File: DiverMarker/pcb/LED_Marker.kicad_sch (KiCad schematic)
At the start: 27 parts, among them IC101 PIC16LF15313, J101 SKEDD6, Q100 BST-52, Q101 BST-52, SW101 MK15-C2

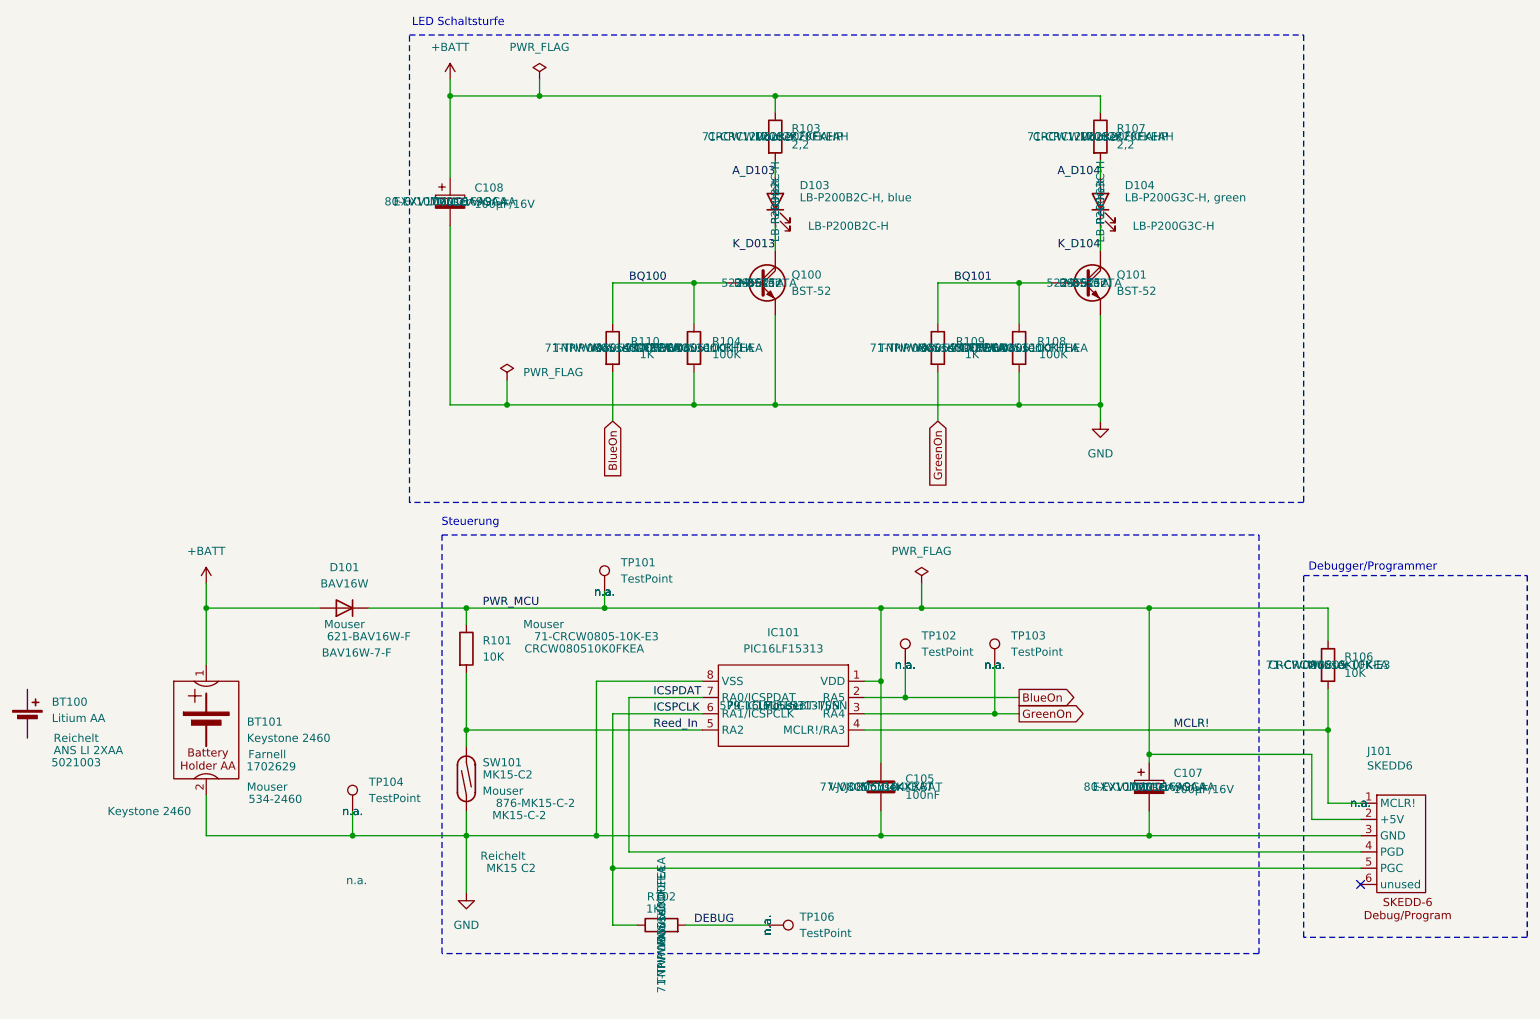
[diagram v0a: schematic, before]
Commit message: Working on BON
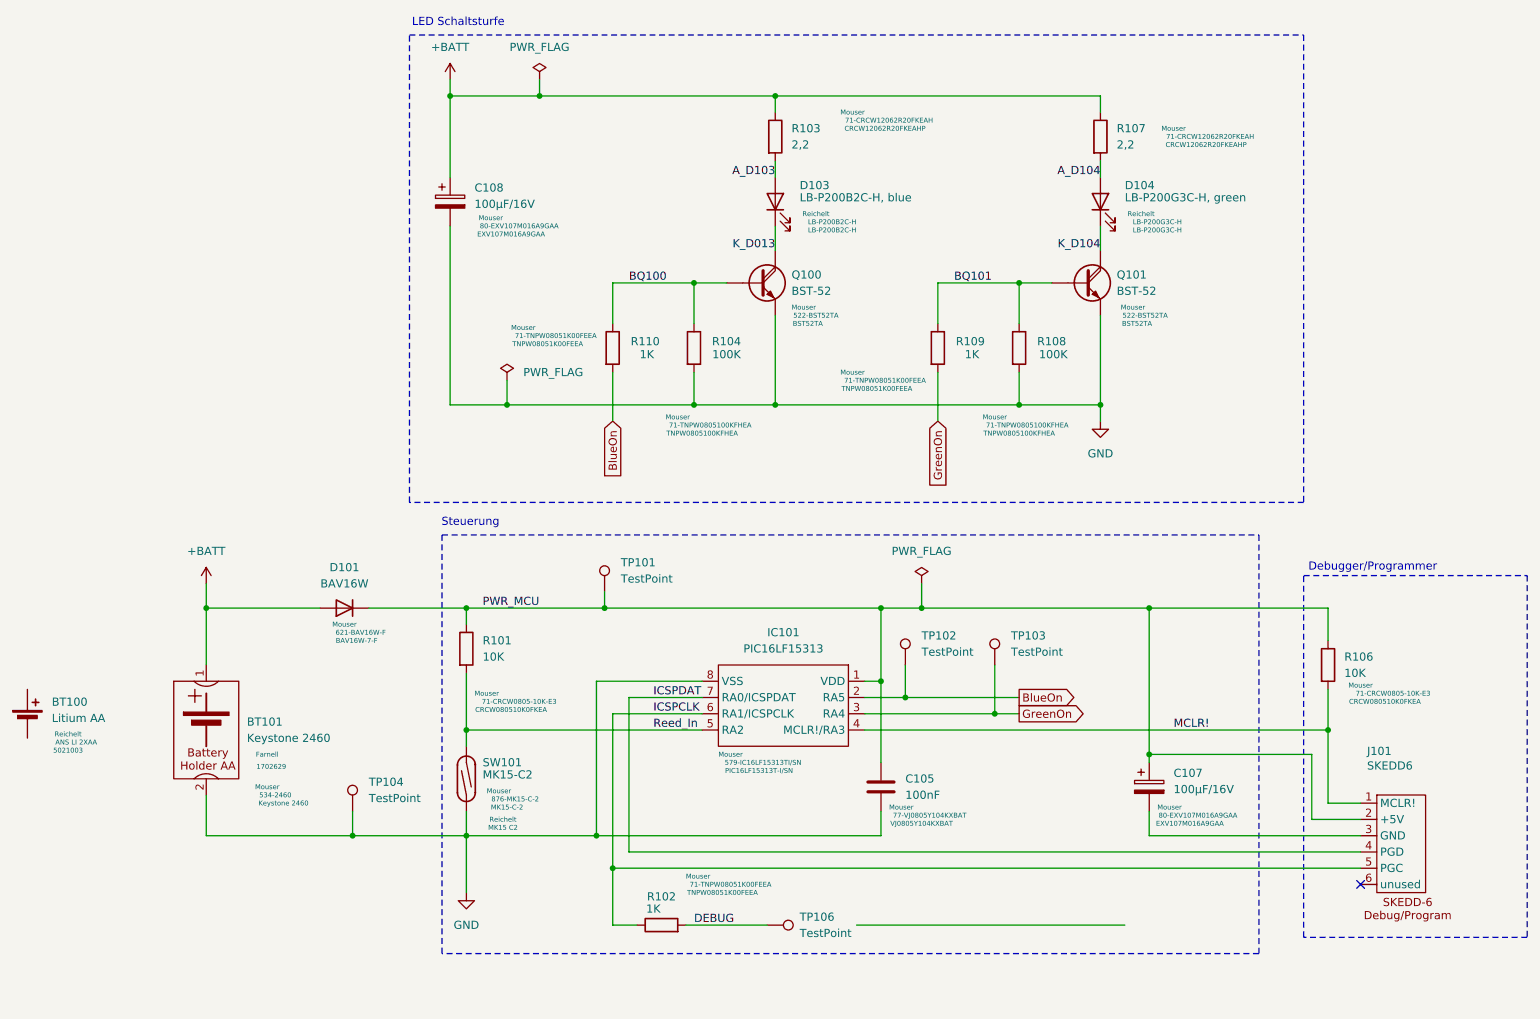
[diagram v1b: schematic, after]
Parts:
- J101, TP101, TP102, TP103, TP104, TP106: Distributor_1 n.a. -> (none)
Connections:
- net GND: no longer C107.2, J101.3 (GND)
- new net: C107.2, J101.3 (GND)
